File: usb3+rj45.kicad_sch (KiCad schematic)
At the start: 63 parts, among them J1 Amphenol_RJE361882415, T1 Choke_SRF2012A-801Y, T2 Choke_SRF2012A-801Y, T3 Choke_SRF2012A-801Y, T4 Choke_SRF2012A-801Y, T5 Trans_SM453229-381N7Y, T6 Trans_SM453229-381N7Y, T7 Trans_SM453229-381N7Y, T8 Trans_SM453229-381N7Y, U1 ESD204DQAR, U2 ESD204DQAR, U3 AP22615A_TSOT26, U4 AP22615A_TSOT26

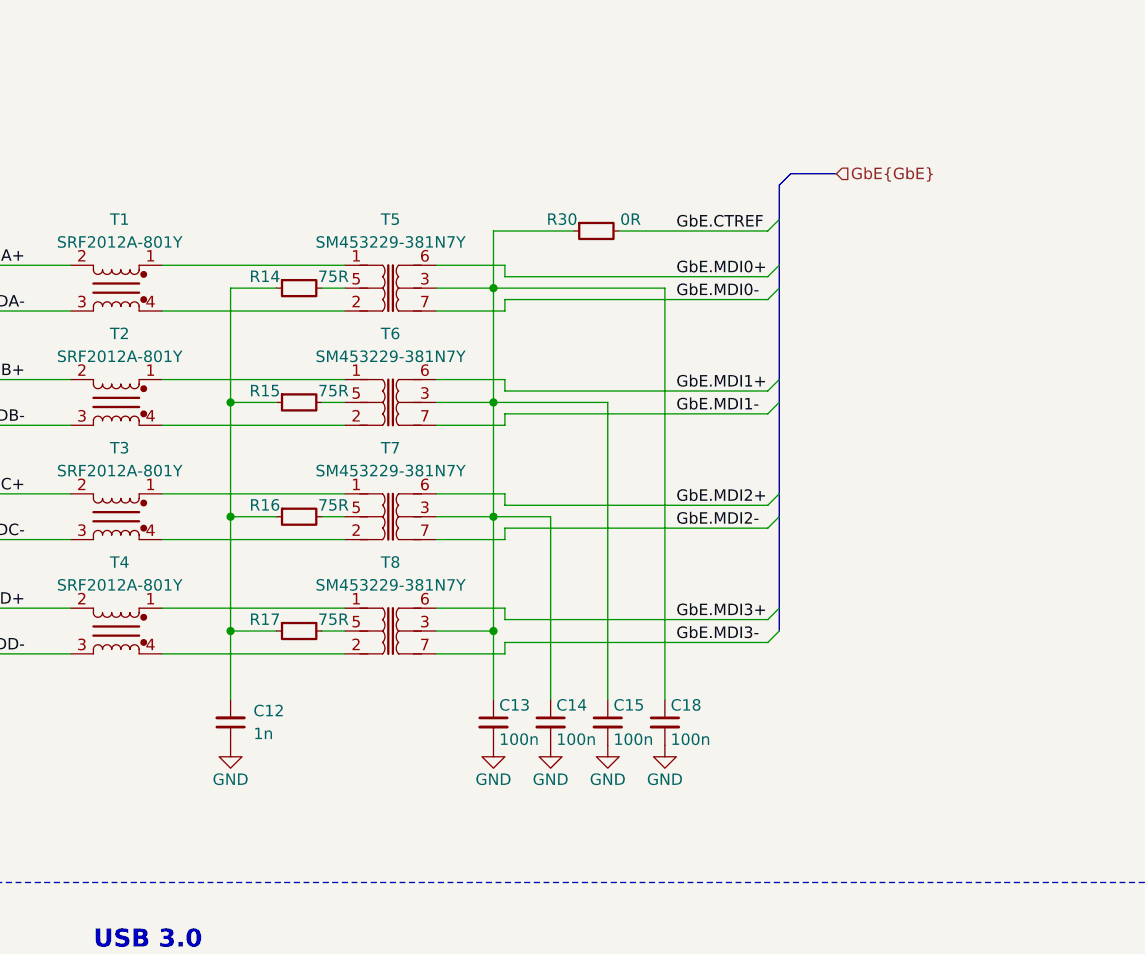
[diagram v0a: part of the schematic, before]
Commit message: [#65840] Roughly route PCIe, GbE
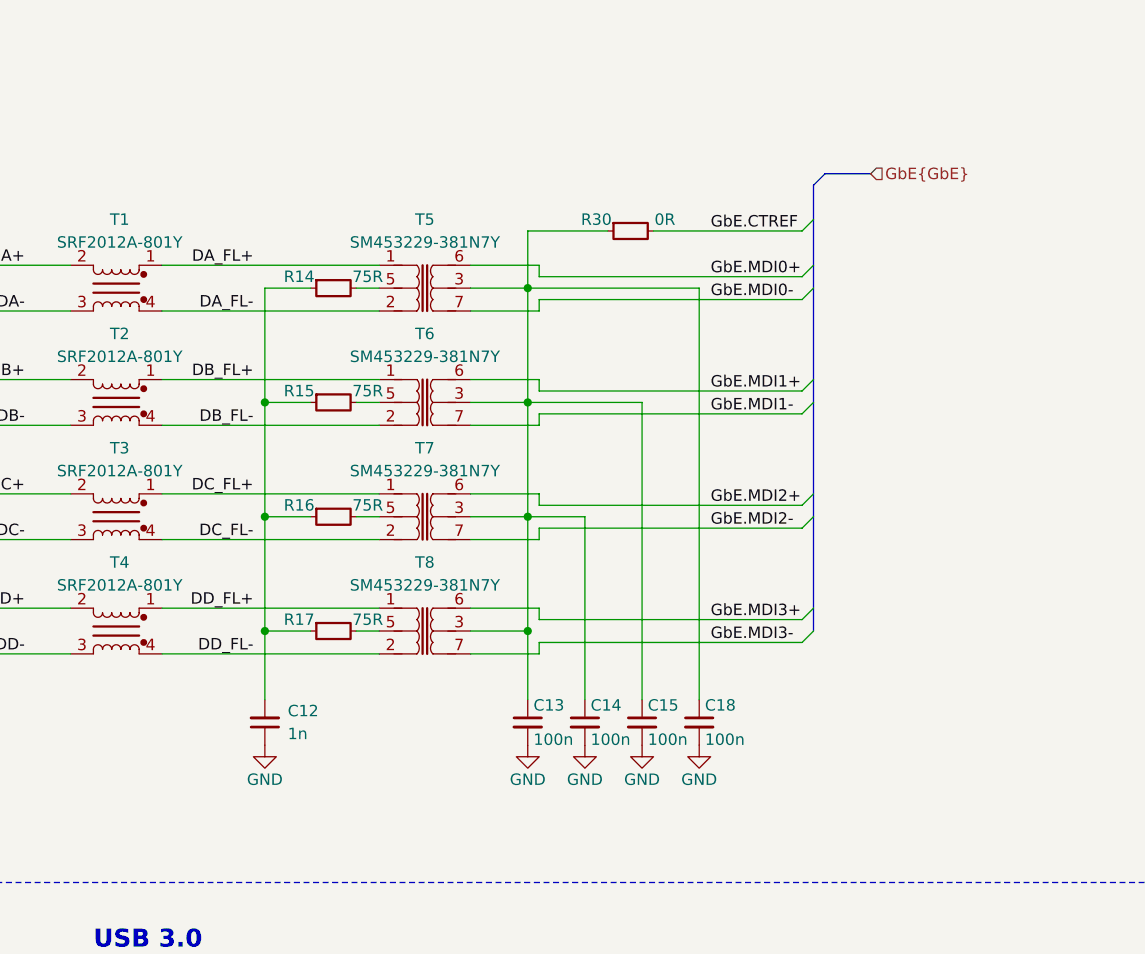
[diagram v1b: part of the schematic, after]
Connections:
- net DC_FL+: now reaches T3.1, T7.1
- net DC_FL-: now reaches T3.4, T7.2
- net DD_FL+: now reaches T4.1, T8.1
- net DD_FL-: now reaches T4.4, T8.2
- net DA_FL+: now reaches T1.1, T5.1
- net DA_FL-: now reaches T1.4, T5.2
- net DB_FL+: now reaches T2.1, T6.1
- net DB_FL-: now reaches T2.4, T6.2
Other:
- moved on the sheet: C12, C13, C14, C15, C18, R14, R15, R16, R17, R30, T5, T6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
